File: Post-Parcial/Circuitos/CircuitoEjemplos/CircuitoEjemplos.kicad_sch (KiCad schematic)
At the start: 7 parts

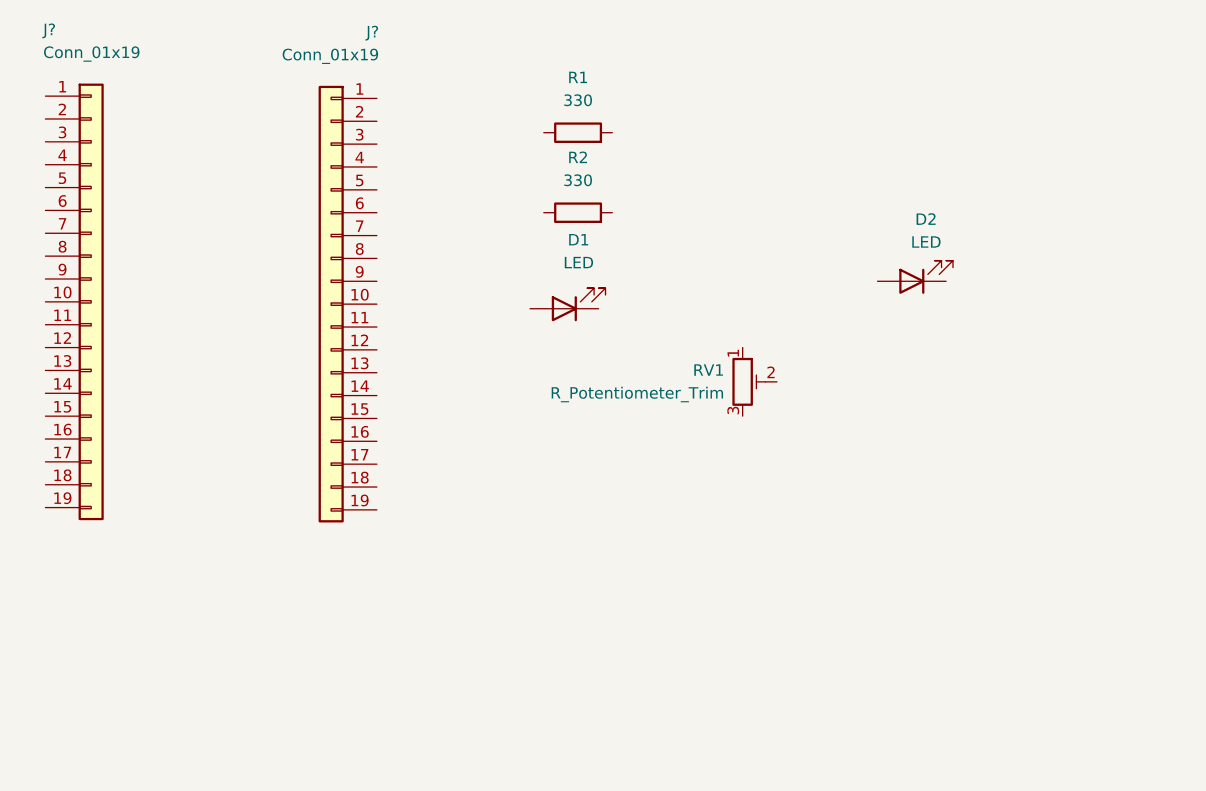
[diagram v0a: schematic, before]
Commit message: Cambio de estructura
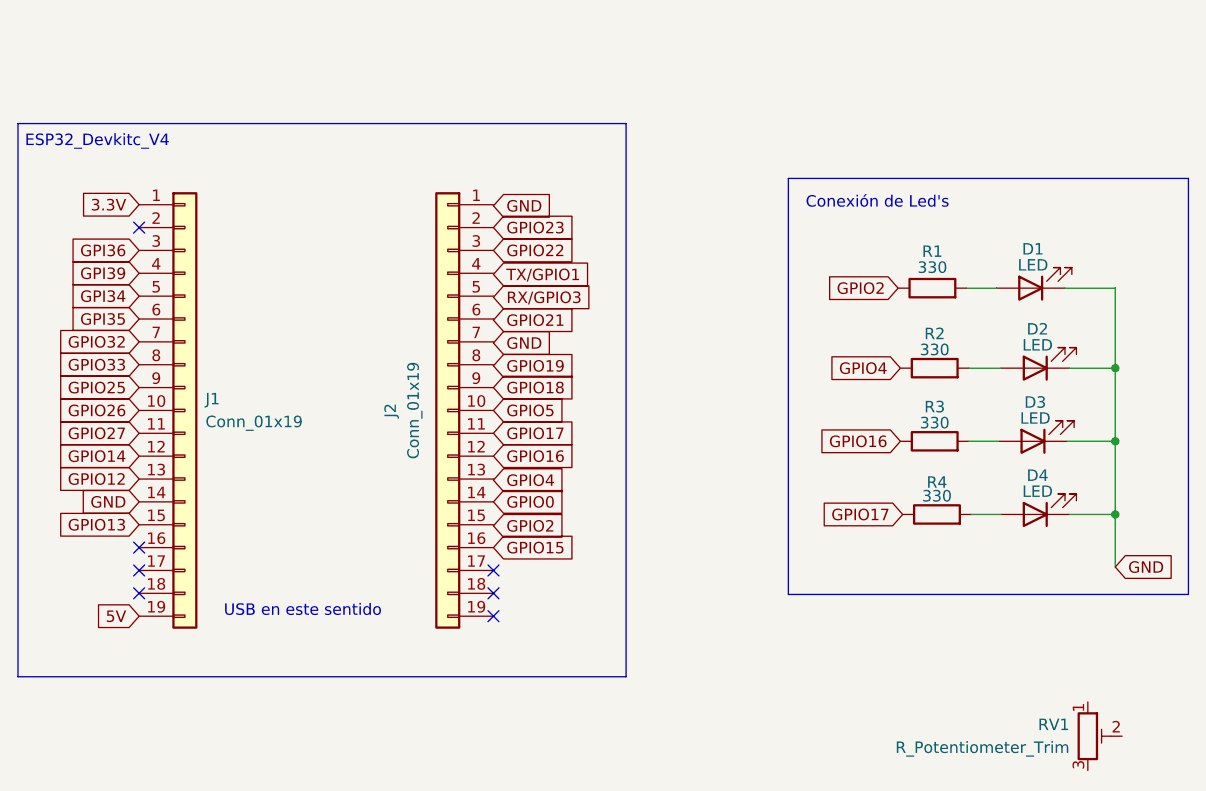
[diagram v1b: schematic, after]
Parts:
- removed J? (x2): Conn_01x19, symbol Connector_Generic:Conn_01x19
- added D3, D4: LED, symbol Device:LED
- added J1, J2: Conn_01x19, Connector_PinSocket_2.54mm:PinSocket_1x19_P2.54mm_Vertical, symbol Connector_Generic:Conn_01x19
- added R3, R4: 330, symbol Device:R
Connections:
- net GPIO4: now reaches R2.1
- net GPIO4: now also J2.13 (Pin_13)
- net at R2.2: now also D2.2 (A)
- net GND: now reaches D2.1 (K)
- net GND: now also D1.1 (K), D3.1 (K), D4.1 (K), J1.14 (Pin_14), J2.1 (Pin_1), J2.7 (Pin_7)
- net GPIO2: now reaches R1.1
- net GPIO2: now also J2.15 (Pin_15)
- net at R1.2: now also D1.2 (A)
- new net: D4.2 (A), R4.2
- new net: D3.2 (A), R3.2
- new net 3.3V: J1.1 (Pin_1)
- new net 5V: J1.19 (Pin_19)
- new net GPI34: J1.5 (Pin_5)
- new net GPI35: J1.6 (Pin_6)
- new net GPI36: J1.3 (Pin_3)
- new net GPI39: J1.4 (Pin_4)
- new net GPIO0: J2.14 (Pin_14)
- new net GPIO12: J1.13 (Pin_13)
- new net GPIO13: J1.15 (Pin_15)
- new net GPIO14: J1.12 (Pin_12)
- new net GPIO15: J2.16 (Pin_16)
- new net GPIO16: J2.12 (Pin_12), R3.1
- new net GPIO17: J2.11 (Pin_11), R4.1
- new net GPIO18: J2.9 (Pin_9)
- new net GPIO19: J2.8 (Pin_8)
- new net GPIO21: J2.6 (Pin_6)
- new net GPIO22: J2.3 (Pin_3)
- new net GPIO23: J2.2 (Pin_2)
- new net GPIO25: J1.9 (Pin_9)
- new net GPIO26: J1.10 (Pin_10)
- new net GPIO27: J1.11 (Pin_11)
- new net GPIO32: J1.7 (Pin_7)
- new net GPIO33: J1.8 (Pin_8)
- new net GPIO5: J2.10 (Pin_10)
- new net RX/GPIO3: J2.5 (Pin_5)
- new net TX/GPIO1: J2.4 (Pin_4)
- no-connect marks 0 -> 7
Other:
- note added: "Conexión de Led's"
- note added: "ESP32_Devkitc_V4"
- note added: "USB en este sentido"
- moved on the sheet: D1, R1, R2, RV1
